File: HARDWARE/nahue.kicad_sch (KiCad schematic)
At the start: 41 parts, among them J2 Screw_Terminal_01x03, J4 Screw_Terminal_01x03, J5 Screw_Terminal_01x03, K1 JQC-3FF-005-1Z, K2 JQC-3FF-005-1Z, K3 JQC-3FF-005-1Z, K4 JQC-3FF-005-1Z, Q1 MMBT3904, Q2 MMBT3904, Q3 MMBT3904, Q4 MMBT3904, U1 PC817, U2 PC817, U3 PC817, U4 PC817, U6 LM7805_TO220

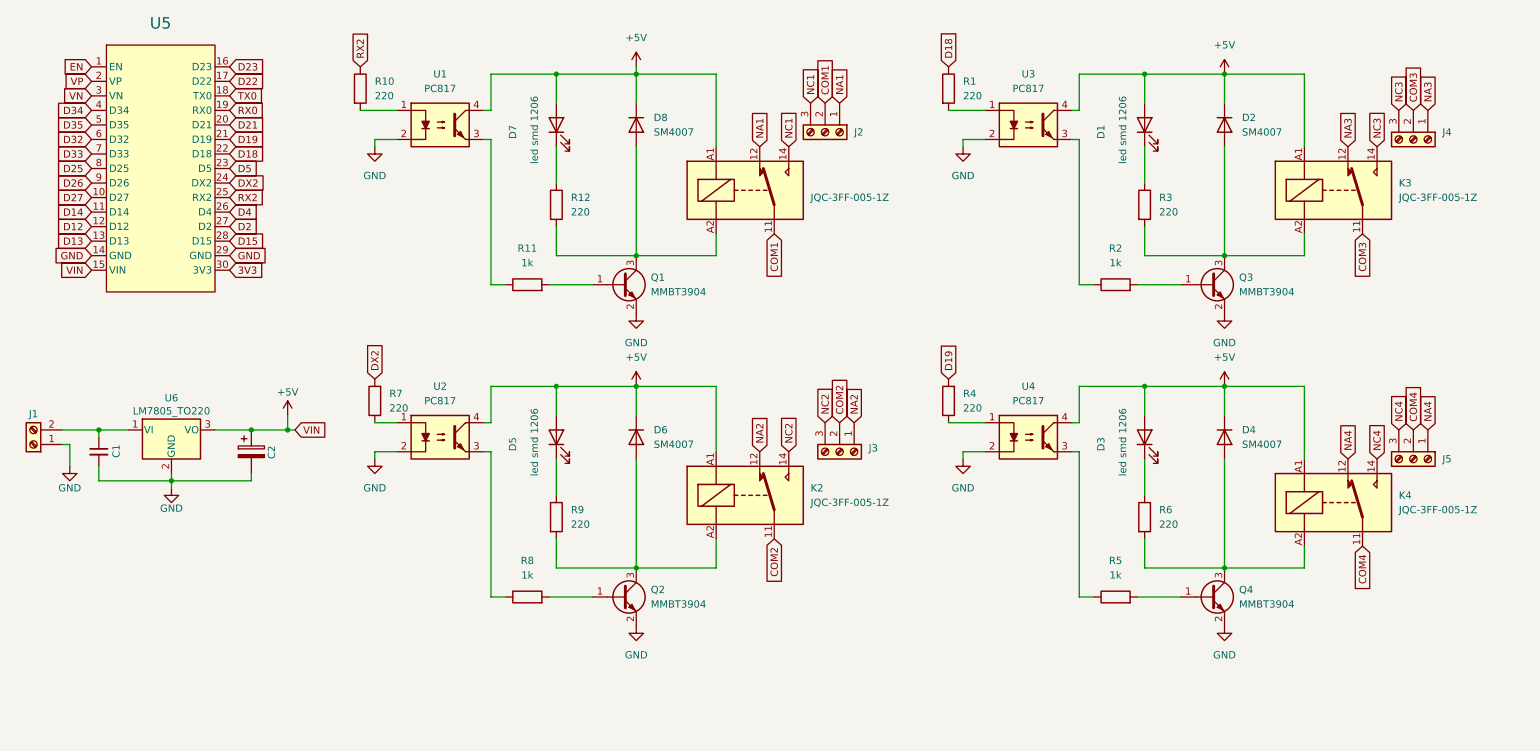
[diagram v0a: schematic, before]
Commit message: retoques del kicad
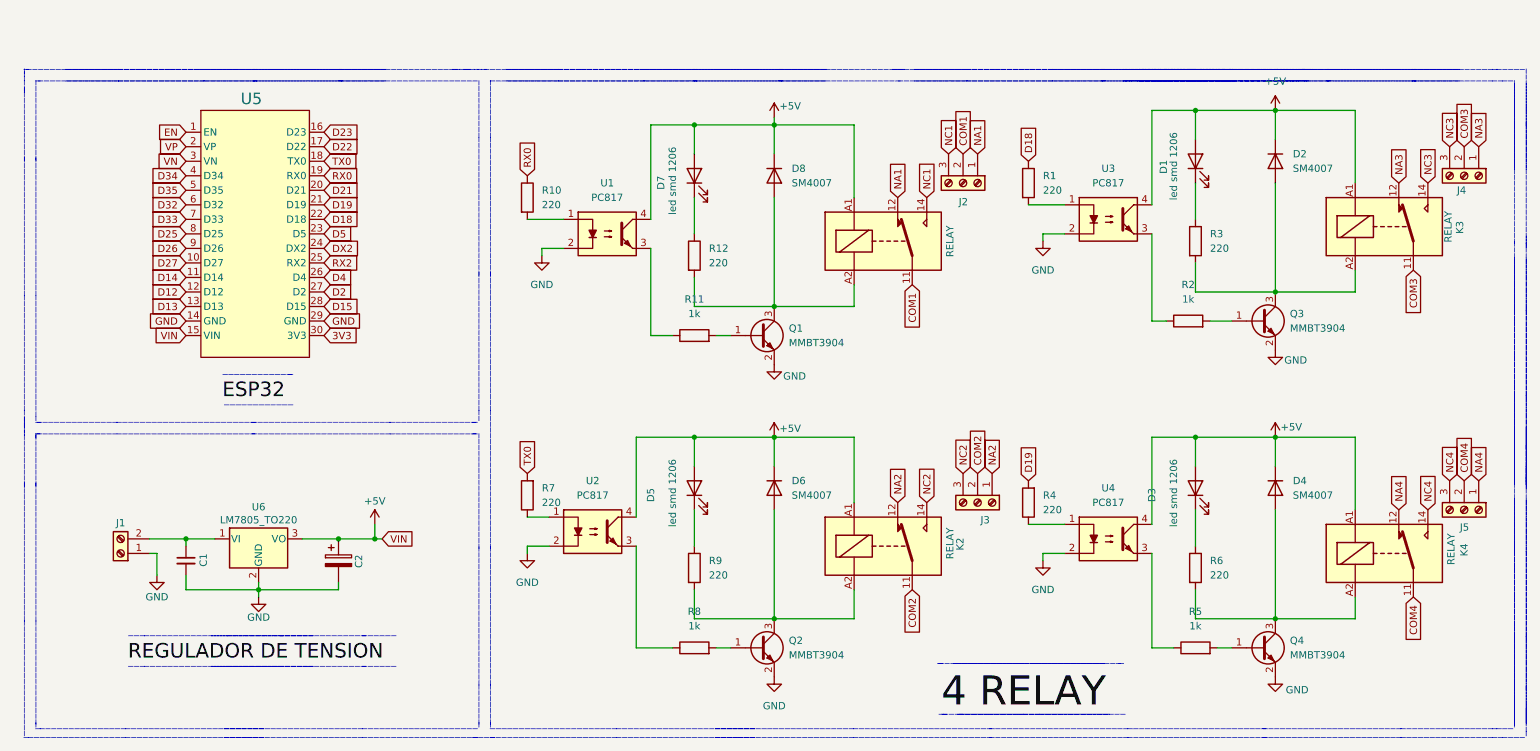
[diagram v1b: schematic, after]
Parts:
- K1, K2, K3, K4: value JQC-3FF-005-1Z -> RELAY
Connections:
- net DX2: no longer R7.2
- net RX0: now also R10.1
- net RX2: no longer R10.1
- net TX0: now also R7.2
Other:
- note added: "_"
- moved on the sheet: C1, C2, D1, D2, D3, D4, D5, D6, D7, D8, J1, J2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
